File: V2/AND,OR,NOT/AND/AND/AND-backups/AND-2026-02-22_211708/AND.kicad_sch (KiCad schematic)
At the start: 15 parts, among them J1 Conn_01x03_Socket, J3 Conn_01x03_Socket, J4 Conn_01x03_Socket, Q1 BSS138, Q2 BSS138, Q3 BSS138, U1 74LVC1G08

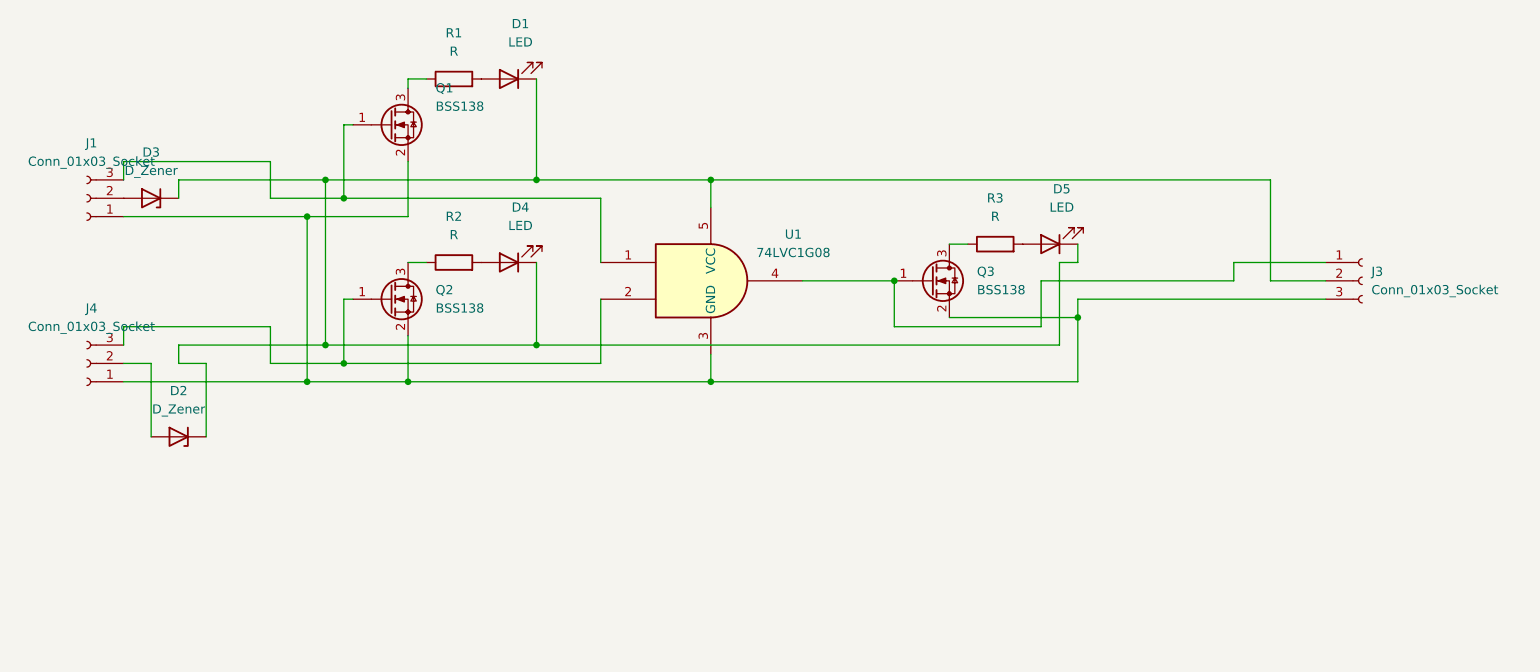
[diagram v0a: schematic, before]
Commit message: fertige Schematik
fertige Schematik
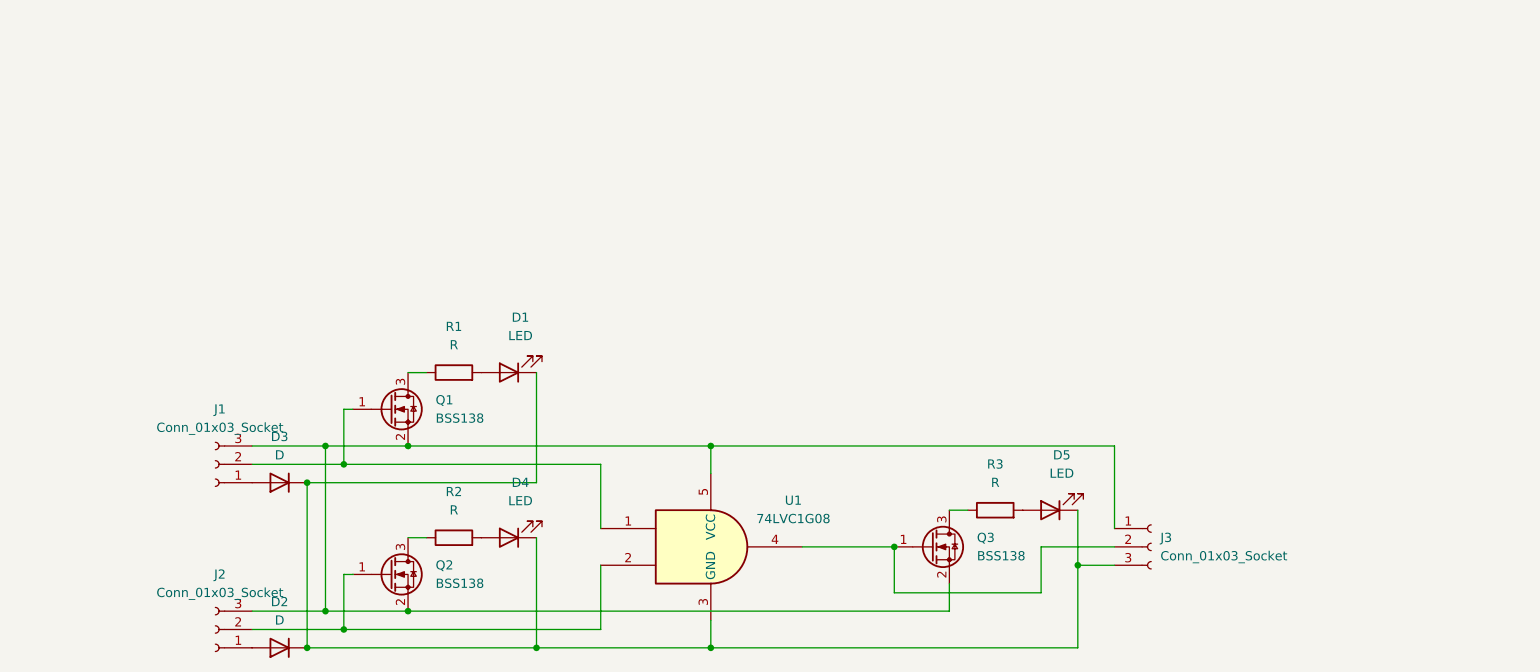
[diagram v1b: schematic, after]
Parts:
- removed D2, D3: D_Zener, Diode_SMD:D_0201_0603Metric, symbol Device:D_Zener
- removed J4: Conn_01x03_Socket, Connector_PinSocket_2.54mm:PinSocket_1x03_P2.54mm_Horizontal, symbol Connector:Conn_01x03_Socket
- added D2, D3: D, Diode_SMD:D_0201_0603Metric, symbol Device:D
- added J2: Conn_01x03_Socket, Connector_PinSocket_2.54mm:PinSocket_1x03_P2.54mm_Horizontal, symbol Connector:Conn_01x03_Socket
- D1, D4, D5: footprint LED_SMD:LED_1206_3216Metric -> Connector_JST:JST_ZH_S3B-ZR-SM4A-TF_1x03-1MP_P1.50mm_Horizontal
- U1: footprint Package_TO_SOT_SMD:SOT-353_SC-70-5 -> Package_TO_SOT_SMD:Texas_DDF0008A_SOT-8_1.6x2.9mm_P0.65mm
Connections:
- net at Q3.1 (G), U1.4: now also J3.2 (Pin_2); no longer J3.1 (Pin_1)
- net at D1.1 (K), D4.1 (K), D5.1 (K): now also J3.3 (Pin_3), U1.3 (GND), D2.1 (K), D3.1 (K); no longer J3.2 (Pin_2), U1.5 (VCC)
- net at Q1.2 (S), Q2.2 (S), Q3.2 (S): now also J1.3 (Pin_3), J3.1 (Pin_1), U1.5 (VCC), J2.3 (Pin_3); no longer J1.1 (Pin_1), J3.3 (Pin_3), U1.3 (GND)
- net at Q2.1 (G), U1.2: now also J2.2 (Pin_2)
- net at J1.2 (Pin_2): now also Q1.1 (G), U1.1
- new net: D3.2 (A), J1.1 (Pin_1)
- new net: D2.2 (A), J2.1 (Pin_1)
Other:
- moved on the sheet: D1, D4, D5, J1, J3, Q1, Q2, Q3, R1, R2, R3, U1
